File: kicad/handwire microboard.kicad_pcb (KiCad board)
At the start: 2 copper layers, 34.1 x 47.3 mm, 10 parts, among them J1 ProMicro18pin, J2 ProMicro18pin, SW1 SW_Push, T1 AudioJack4, T2 AudioJack4, T3 AudioJack4, T4 AudioJack4, U1 ProMicro

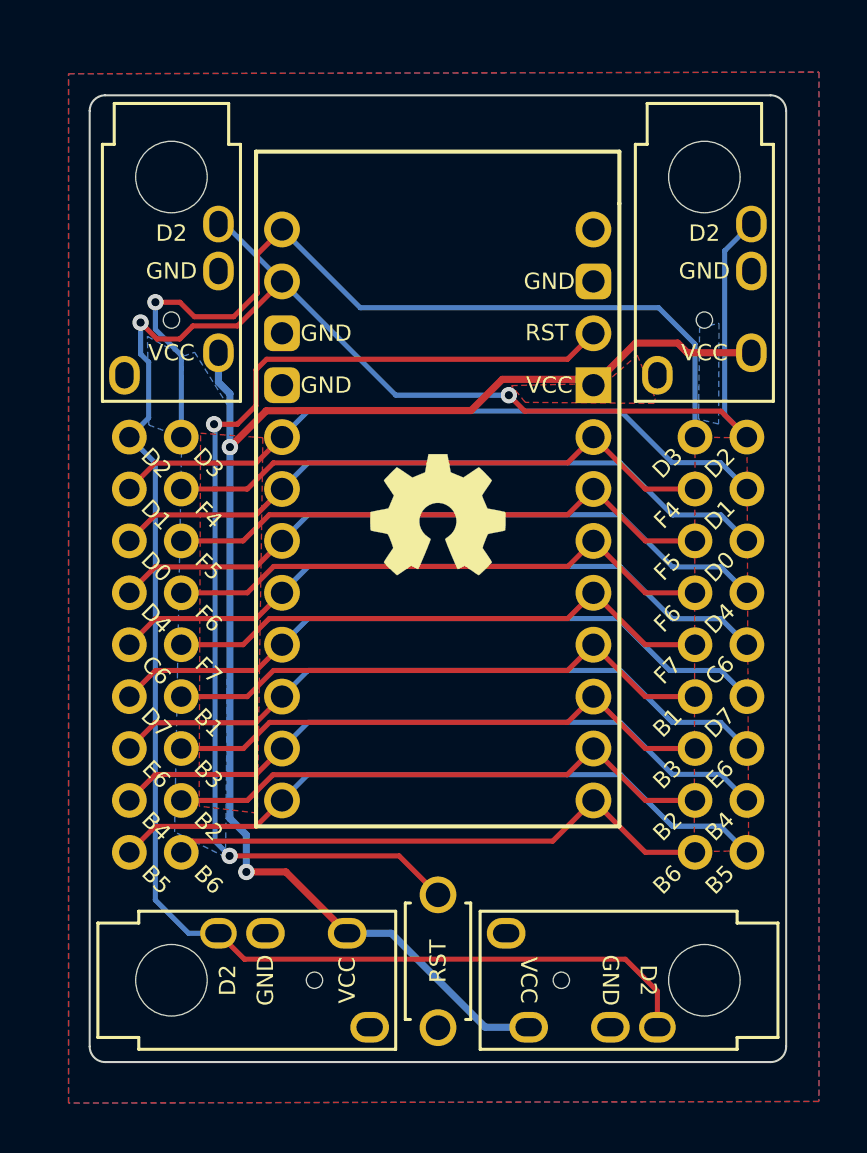
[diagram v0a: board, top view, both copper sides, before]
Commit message: new design
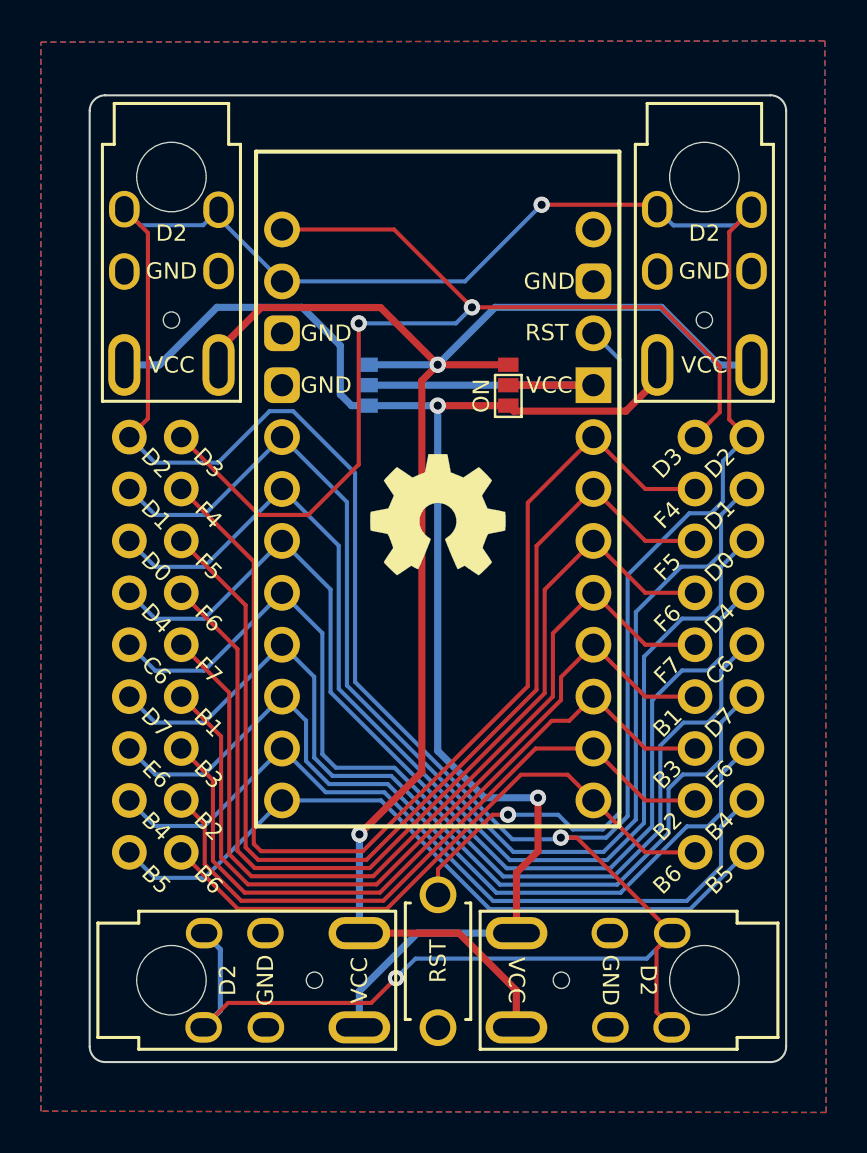
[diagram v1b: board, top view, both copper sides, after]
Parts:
- added ON: Jumper_Fside, DreaM117er-keebLibrary:SolderJumper-3_P1.3mm_Open_Pad0.7.x1.0mm_NumberLabels, F.Cu at (38.3, 32.1)
- added ON: Jumper_Bside, DreaM117er-keebLibrary:SolderJumper-3_P1.3mm_Open_Pad0.7.x1.0mm_NumberLabels, B.Cu at (31.5, 32.1)
- T1, T2, T3, T4: footprint DreaM117er-keebLibrary:TRRS-PJ-320A -> DreaM117er-keebLibrary:TRRS-PJ-320A, dual side
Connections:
- T1 pad 1: VCC -> A
- T1 pad 4: unconnected-(T1-S/No-Pad4) -> B
- T2 pad 1: VCC -> A
- T2 pad 4: unconnected-(T2-S/No-Pad4) -> B
- T3 pad 1: VCC -> A
- T3 pad 4: unconnected-(T3-S/No-Pad4) -> B
- T4 pad 1: VCC -> A
- T4 pad 4: unconnected-(T4-S/No-Pad4) -> B
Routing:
- net A: track 0.00 -> 78.1 mm, vias 0 -> 2
- net B: track 0.00 -> 72.6 mm, vias 0 -> 2
- net D2: track 107.5 -> 164.7 mm, vias 2 -> 3
- net VCC: track 71.0 -> 15.2 mm, vias 2 -> 0
- net F4: track 27.2 -> 55.3 mm
- net D1: track 33.4 -> 60.4 mm
- net F5: track 27.2 -> 51.2 mm
- net D0: track 33.4 -> 56.3 mm
- net F6: track 27.2 -> 47.2 mm
- net D4: track 33.4 -> 52.2 mm
- net RESET: track 53.9 -> 35.9 mm, vias 2 -> 1
- net C6: track 33.4 -> 49.8 mm
- net F7: track 27.2 -> 43.1 mm
- net D7: track 33.4 -> 45.7 mm
- net B1: track 27.2 -> 39.0 mm
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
